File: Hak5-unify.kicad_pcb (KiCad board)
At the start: 2 copper layers, 26 x 17.5 mm, 4 parts, among them J1 Conn_01x02, J2 Conn_01x03, U1 Unify-Nano

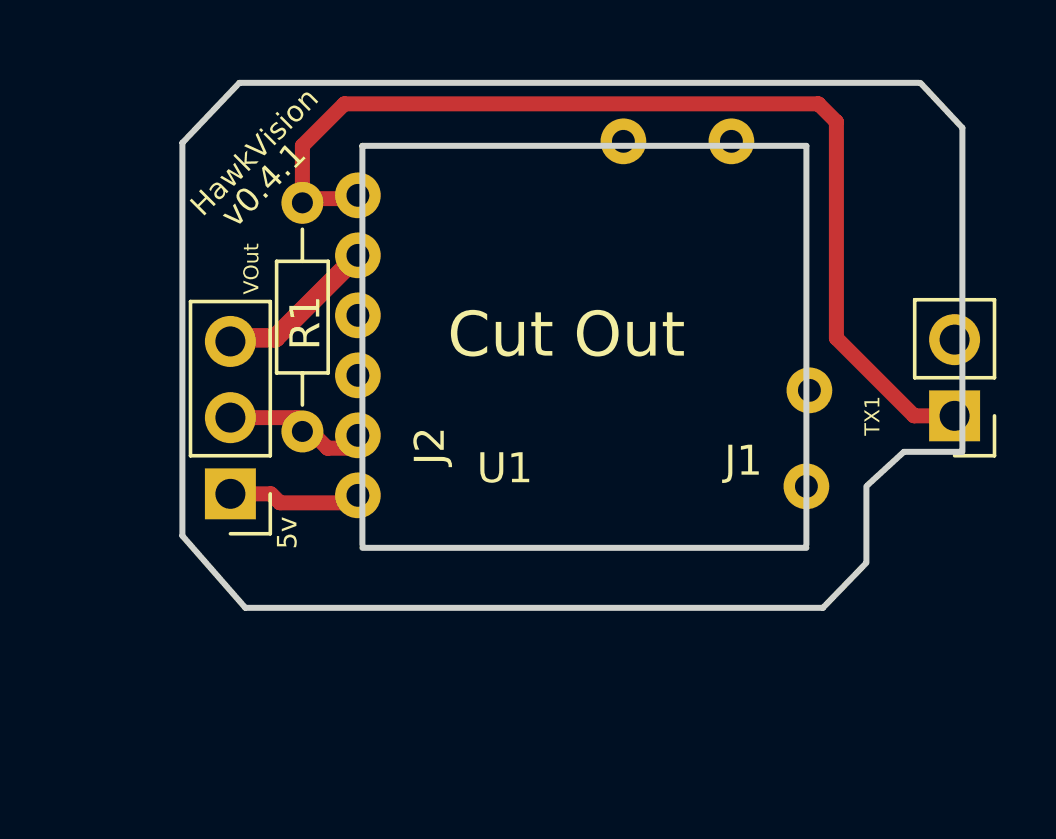
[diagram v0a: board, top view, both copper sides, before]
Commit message: v0.6.0
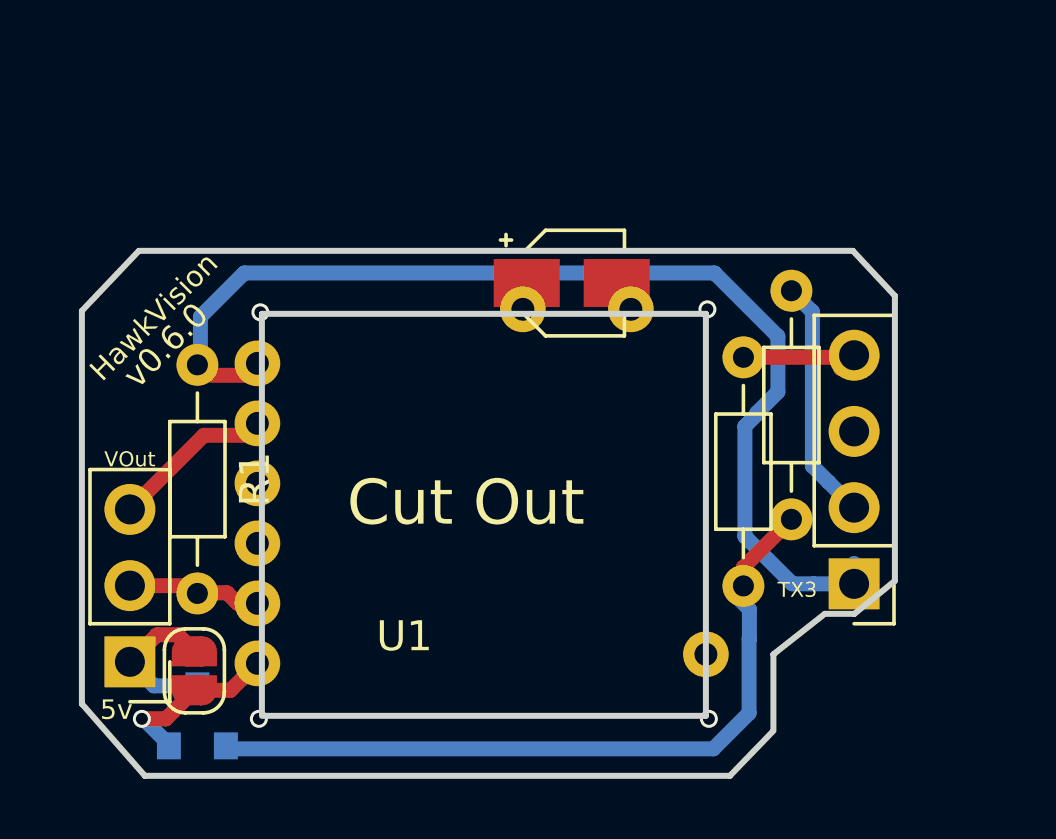
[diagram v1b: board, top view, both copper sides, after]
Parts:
- added JP1: SolderJumper_2_Open, Jumper:SolderJumper-2_P1.3mm_Open_RoundedPad1.0x1.5mm, F.Cu at (100.4, 102.1)
- added Q2: PMV65UNER, Package_TO_SOT_SMD:SOT-23, B.Cu at (100.5, 103.6)
- added R2: 10K, Resistor_THT:R_Axial_DIN0204_L3.6mm_D1.6mm_P7.62mm_Horizontal, F.Cu at (118.7, 91.7)
- added R3: 10K, Resistor_THT:R_Axial_DIN0204_L3.6mm_D1.6mm_P7.62mm_Horizontal, F.Cu at (120.3, 97.0)
- added SW1: SW_Push, Capacitor_SMD:CP_Elec_3x5.3, F.Cu at (113.0, 89.2)
- J1: value Conn_01x02 -> Conn_01x04; footprint Pin_Headers:Pin_Header_Straight_1x02_Pitch2.54mm -> Pin_Headers:Pin_Header_Straight_1x04_Pitch2.54mm
- R1: value R -> 10K; footprint Resistors_ThroughHole:R_Axial_DIN0204_L3.6mm_D1.6mm_P7.62mm_Horizontal -> Resistor_THT:R_Axial_DIN0204_L3.6mm_D1.6mm_P7.62mm_Horizontal
- moved J1 6.53 mm to (122.4, 99.2)
- moved J2 6.53 mm to (98.2, 101.8)
- moved U1 6.53 mm to (102.8, 103.3)
- moved R1 6.44 mm to (100.5, 91.9)
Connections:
- J1 pad 2: Net-(J1-Pad2) -> RX
- U1 pad 6: +5V -> Net-(JP1-Pad1)
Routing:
- net Net-(Q2-Pad1): track 0.00 -> 24.9 mm
- net RX: track 0.00 -> 8.31 mm
- net Net-(JP1-Pad1): track 0.00 -> 5.35 mm, vias 0 -> 1
- net GND: track 4.77 -> 8.45 mm
- net +5V: track 4.47 -> 5.33 mm
- net Net-(SW1-Pad1): track 0.00 -> 0.66 mm
- net Net-(SW1-Pad2): track 0.00 -> 0.62 mm
- net Net-(J2-Pad3): track 5.42 -> 4.87 mm
- net TX: track 34.8 -> 35.3 mm
- net (no net): vias 0 -> 4
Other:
- board size 26 x 17.5 mm -> 27.1 x 17.5 mm
- board text added: "TX3"
- board text added: "v0.6.0"
- board text removed: "TX1"
- board text removed: "v0.4.1"

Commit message: 0.7.0
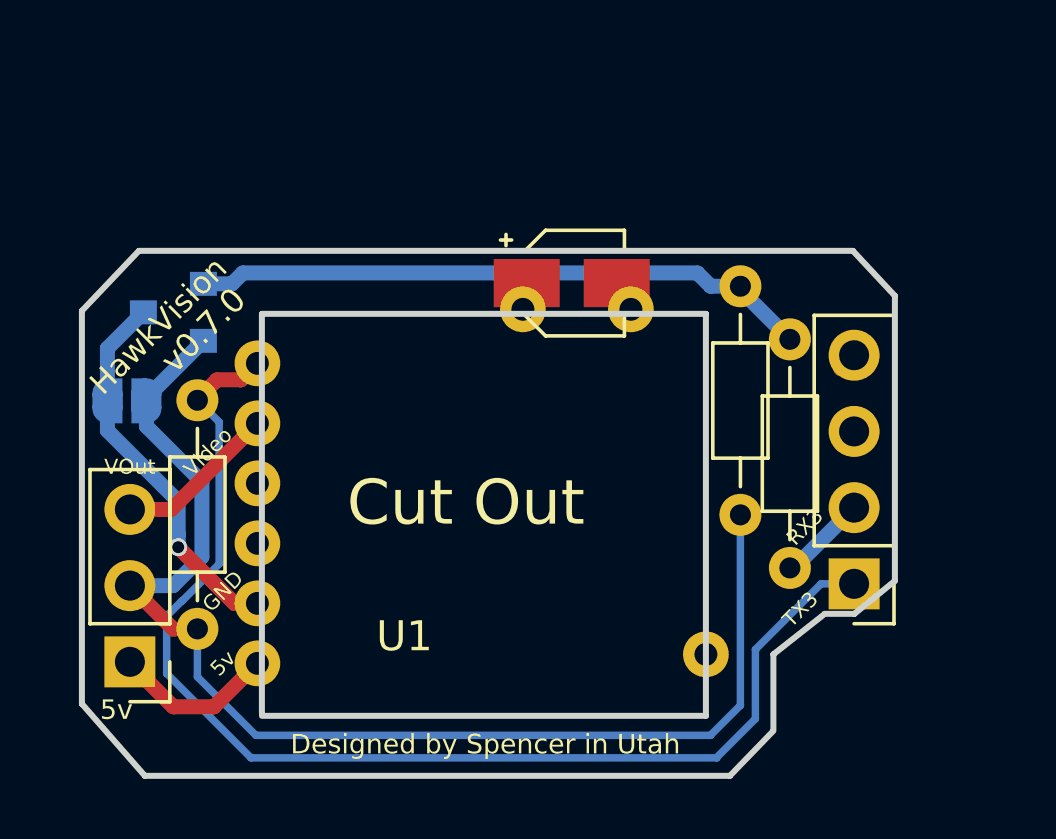
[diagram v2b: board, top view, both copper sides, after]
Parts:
- JP1: moved to B.Cu
- moved Q2 13.5 mm to (99.7, 90.2), turned to 180 degrees
- moved JP1 9.28 mm to (98.2, 93.1), turned to 0 degrees
- moved R3 6.00 mm to (120.2, 91.0), turned to 270 degrees
- moved R2 5.25 mm to (118.6, 96.9), turned to 90 degrees
- moved R1 1.18 mm to (100.5, 93.1)
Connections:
- JP1 pad 2: +5V -> GND
- Q2 pad 2: Net-(JP1-Pad1) -> GND
- Q2 pad 3: +5V -> Net-(JP1-Pad1)
- U1 pad 5: GND -> Net-(JP1-Pad1)
- U1 pad 6: Net-(JP1-Pad1) -> +5V
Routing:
- net GND: track 8.45 -> 42.4 mm
- net Net-(JP1-Pad1): track 5.35 -> 12.4 mm
- net RX: track 8.31 -> 2.97 mm
- net TX: track 35.3 -> 40.0 mm
- net Net-(Q2-Pad1): track 24.9 -> 20.7 mm
- net (no net): vias 4 -> 0
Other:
- board text added: "GND"
- board text added: "RX3"
- board text added: "Video"
- board text added: "v0.7.0"
- board text removed: "v0.6.0"
